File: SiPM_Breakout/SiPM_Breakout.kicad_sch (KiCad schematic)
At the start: 1 part, among them U1 MICROFC-60035-SMT-TR

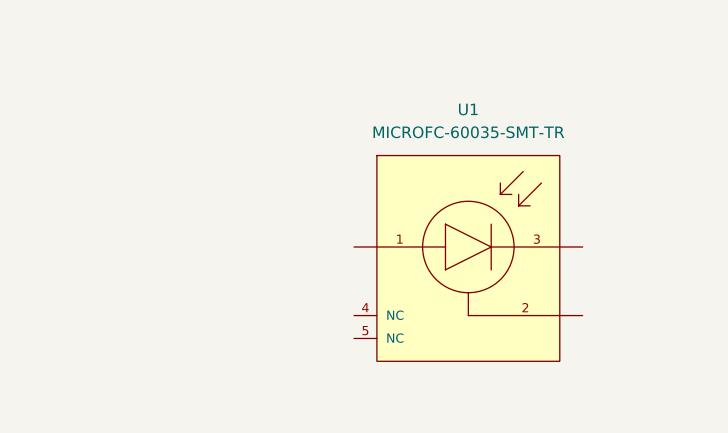
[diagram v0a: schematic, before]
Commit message: Finished Annotations + Completed PCB
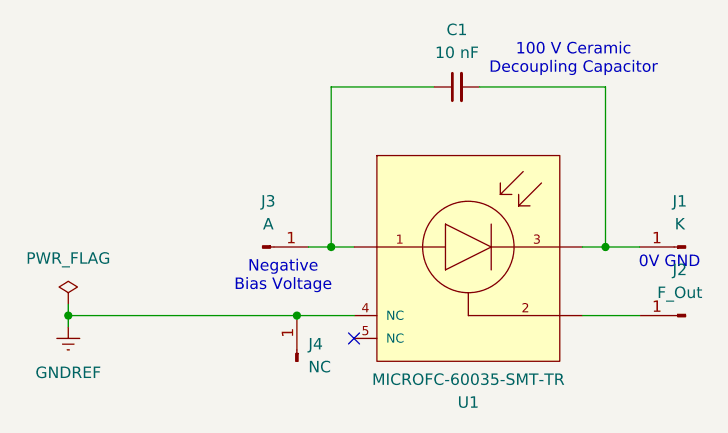
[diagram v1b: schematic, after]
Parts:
- added C1: 10 nF, Capacitor_SMD:C_0805_2012Metric_Pad1.18x1.45mm_HandSolder, symbol Device:C_Small
- added J1: K, Connector_PinHeader_1.00mm:PinHeader_1x01_P1.00mm_Vertical, symbol Connector:Conn_01x01_Pin
- added J2: F_Out, Connector_PinHeader_1.00mm:PinHeader_1x01_P1.00mm_Vertical, symbol Connector:Conn_01x01_Pin
- added J3: A, Connector_PinHeader_1.00mm:PinHeader_1x01_P1.00mm_Vertical, symbol Connector:Conn_01x01_Pin
- added J4: NC, Connector_PinHeader_1.00mm:PinHeader_1x01_P1.00mm_Vertical, symbol Connector:Conn_01x01_Pin
- U1: footprint MICROFC-60035-SMT-TR:ON_Semiconductor-512AG-07_2018-O-MFG -> Onsemi:ON_Semiconductor-512AG-07_2018-O-MFG
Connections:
- net at U1.1 (Anode): now also C1.1, J3.1 (Pin_1)
- net at U1.2 (Fast_Output): now also J2.1 (Pin_1)
- net at U1.3 (Cathode): now also C1.2, J1.1 (Pin_1)
- net GNDREF: now reaches U1.4 (NC)
- net GNDREF: now also J4.1 (Pin_1)
- no-connect marks 0 -> 1
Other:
- note added: "0V GND"
- note added: "100 V Ceramic Decoupling Capacitor"
- note added: "Negative Bias Voltage"
